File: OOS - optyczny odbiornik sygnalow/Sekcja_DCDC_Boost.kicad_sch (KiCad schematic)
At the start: 18 parts, among them U3 AP3015KTR-G1

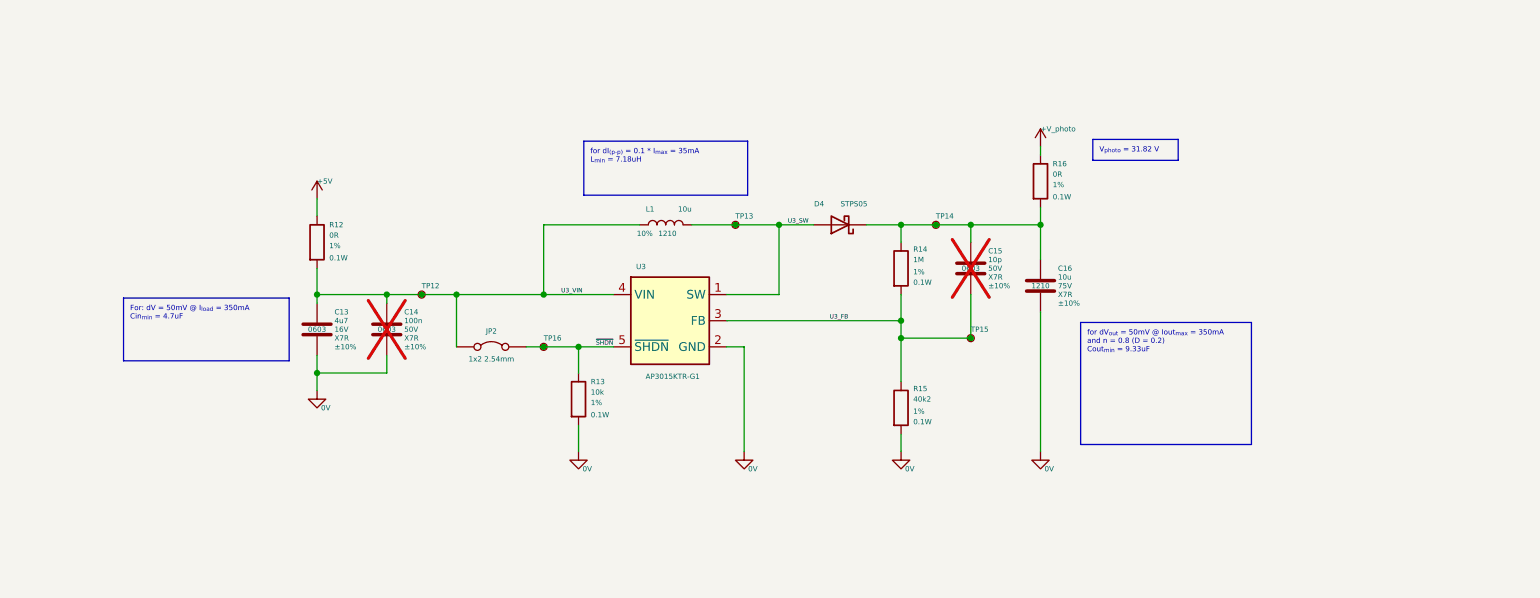
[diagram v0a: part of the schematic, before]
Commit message: Finish Li-Lion section, add for review
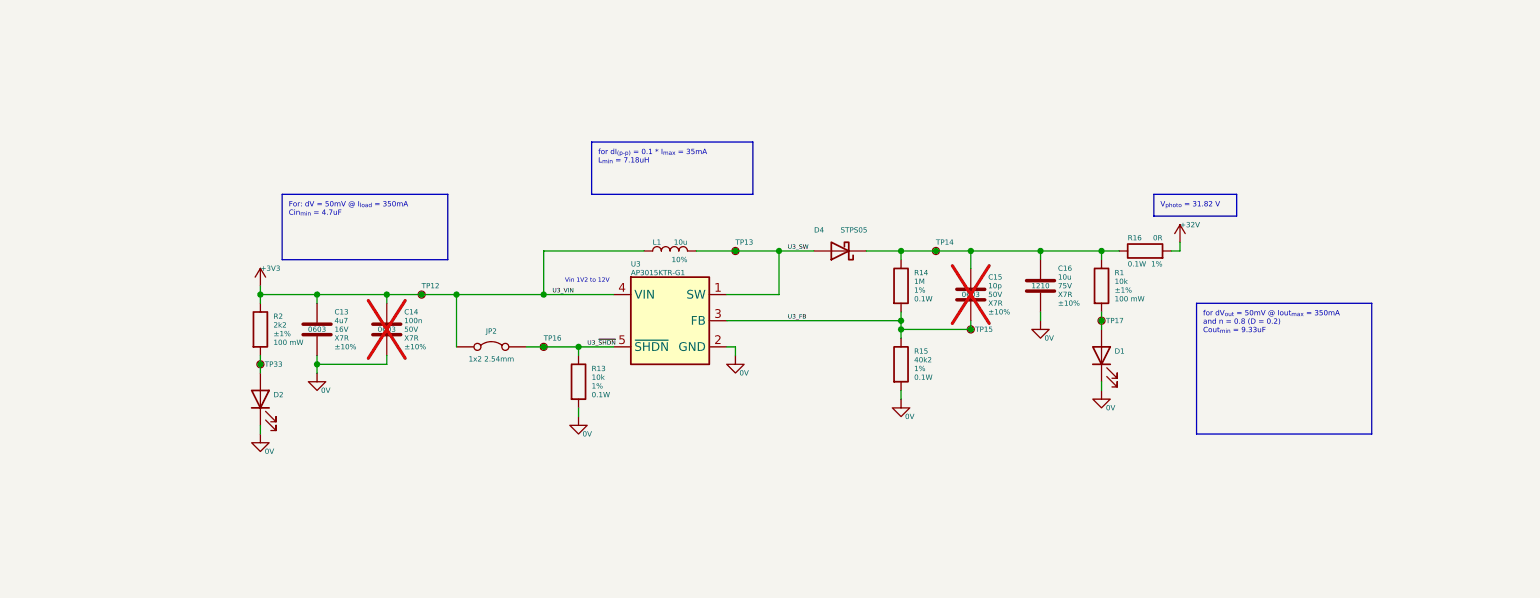
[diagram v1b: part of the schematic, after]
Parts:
- removed R12: 0R, Resistor_SMD:R_0603_1608Metric, symbol Device:R
- added D1, D2: LED, Diode_SMD:D_0603_1608Metric_Pad1.05x0.95mm_HandSolder, symbol Device:LED
- added R1: 10k, Resistor_SMD:R_0603_1608Metric_Pad0.98x0.95mm_HandSolder, symbol Device:R
- added R2: 2k2, Resistor_SMD:R_0603_1608Metric_Pad0.98x0.95mm_HandSolder, symbol Device:R
- added TP17, TP33: TestPoint_Small, TestPoint:TestPoint_Pad_D1.0mm, symbol Connector:TestPoint_Small
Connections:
- net +V_photo is gone; now on an unnamed net: R16.1
- net 0V: now also D1.1 (K), D2.1 (K)
- net at C15.1, C16.1, D4.1 (K)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: now also R1.1; no longer R16.2
- net U3_VIN renamed +3V3
- net +3V3: now also R2.1
- net ~{SHDN} renamed U3_~{SHDN}
- new net: D2.2 (A), R2.2, TP33.1
- new net: D1.2 (A), R1.2, TP17.1
- new net +32V: R16.2
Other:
- note added: "Vin 1V2 to 12V"
- moved on the sheet: C15, D4, L1, R13, R14, R15, R16, TP13, TP14, TP15
